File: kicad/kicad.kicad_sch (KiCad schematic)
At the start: 9 parts, among them Q1 BPW40, Q2 BP103BF, U1 PIC16F18875-E/P, U2 L293D

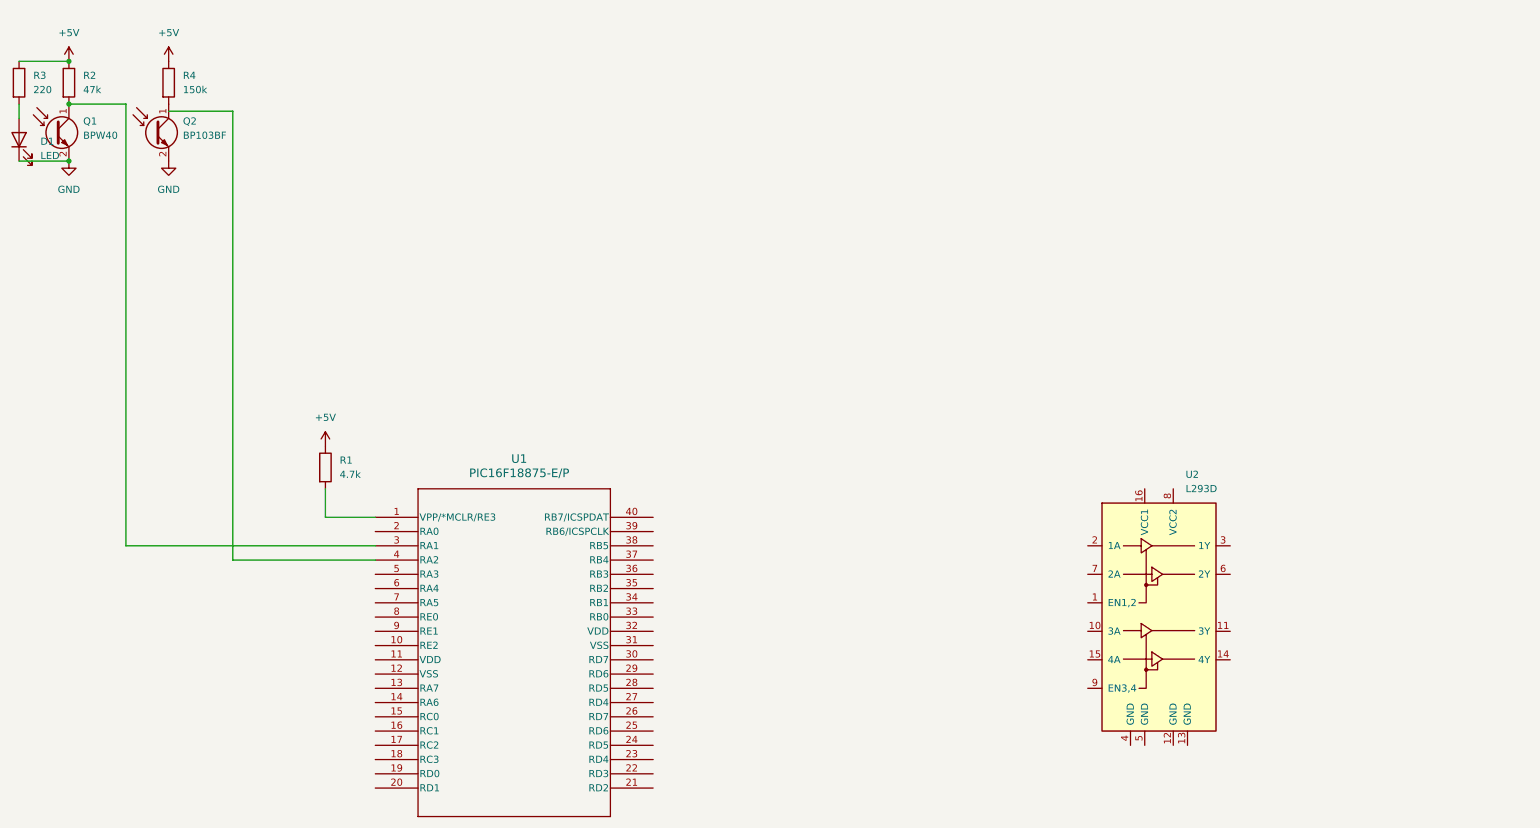
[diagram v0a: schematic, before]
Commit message: finished schematic
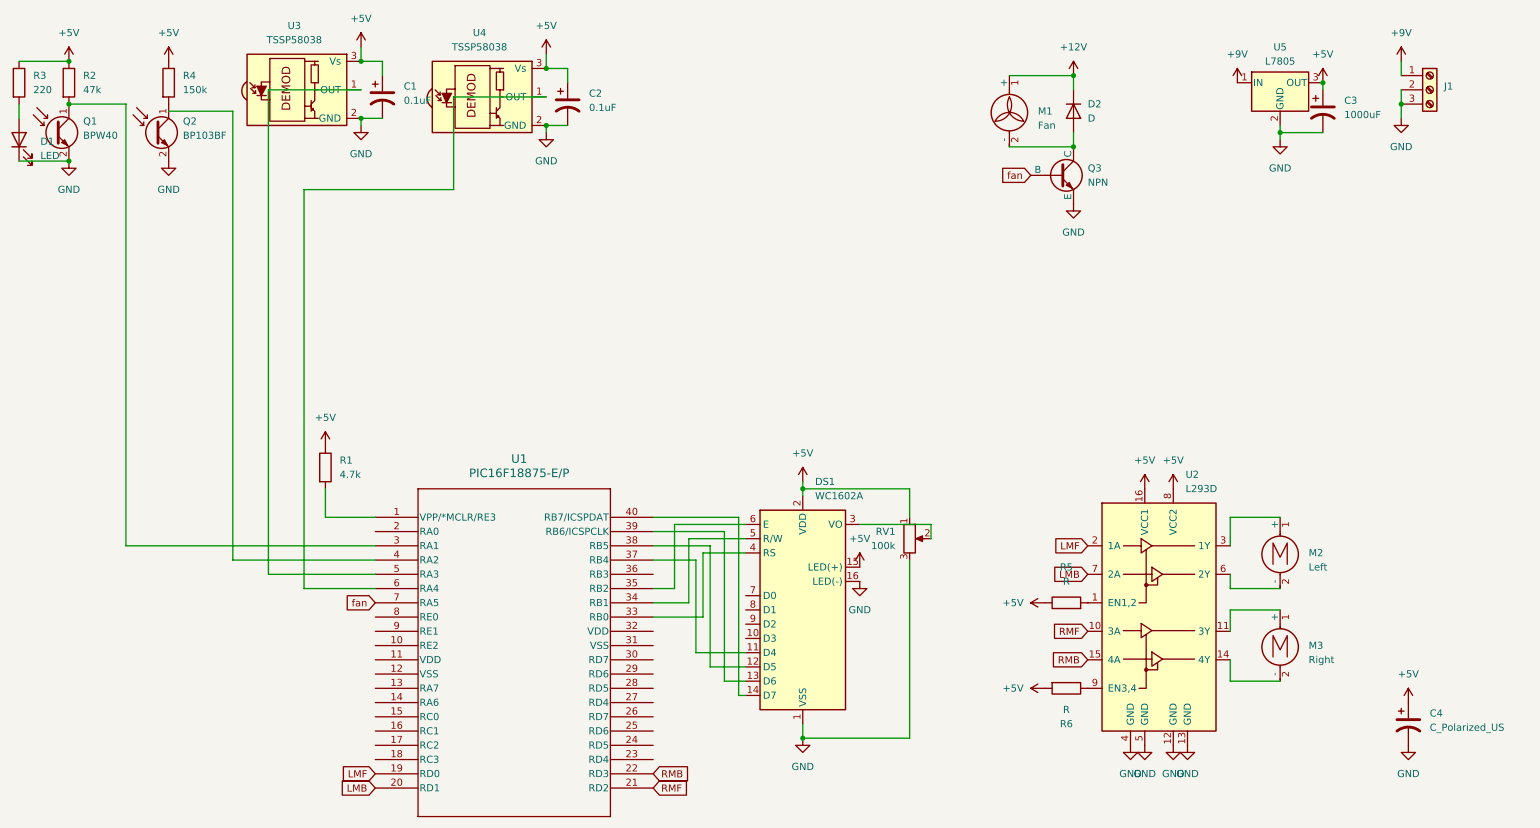
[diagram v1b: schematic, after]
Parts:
- added C1, C2: 0.1uF, symbol Device:C_Polarized_US
- added C3: 1000uF, symbol Device:C_Polarized_US
- added C4: C_Polarized_US, symbol Device:C_Polarized_US
- added D2: D, symbol Device:D
- added DS1: WC1602A, Display:WC1602A, symbol Display_Character:WC1602A
- added J1: ~, symbol Connector:Screw_Terminal_01x03
- added M1: Fan, symbol Motor:Fan
- added M2: Left, symbol Motor:Motor_DC
- added M3: Right, symbol Motor:Motor_DC
- added Q3: NPN, symbol Simulation_SPICE:NPN
- added R5, R6: R, symbol Device:R
- added RV1: 100k, symbol Device:R_Potentiometer
- added U3, U4: TSSP58038, OptoDevice:Vishay_MINICAST-3Pin, symbol Sensor_Proximity:TSSP58038
- added U5: L7805, symbol Regulator_Linear:L7805
- U1: footprint PDIP40_P_MCH -> (none)
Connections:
- net +5V: now also U2.16 (VCC1), U2.8 (VCC2), C1.1, C2.1, C3.1, C4.1, DS1.15 (LED(+)), DS1.2 (VDD), R5.1, R6.2, RV1.1, U3.3 (Vs), U4.3 (Vs), U5.3 (OUT)
- net GND: now also U2.12 (GND), U2.13 (GND), U2.4 (GND), U2.5 (GND), C1.2, C2.2, C3.2, C4.2, DS1.1 (VSS), DS1.16 (LED(-)), J1.2 (Pin_2), J1.3 (Pin_3), Q3.3 (E), RV1.3, U3.2 (GND), U4.2 (GND), U5.2 (GND)
- net at U2.1 (EN1,2): now also R5.2
- net RMF: now reaches U2.10 (3A)
- net RMF: now also U1.21 (RD2)
- net at U2.11 (3Y): now also M3.1 (+)
- net at U2.14 (4Y): now also M3.2 (-)
- net RMB: now reaches U2.15 (4A)
- net RMB: now also U1.22 (RD3)
- net LMF: now reaches U2.2 (1A)
- net LMF: now also U1.19 (RD0)
- net at U2.3 (1Y): now also M2.1 (+)
- net at U2.6 (2Y): now also M2.2 (-)
- net LMB: now reaches U2.7 (2A)
- net LMB: now also U1.20 (RD1)
- net at U2.9 (EN3,4): now also R6.1
- net at U1.33 (RB0): now also DS1.4 (RS)
- net at U1.34 (RB1): now also DS1.5 (R/W)
- net at U1.35 (RB2): now also DS1.6 (E)
- net at U1.37 (RB4): now also DS1.11 (D4)
- net at U1.38 (RB5): now also DS1.12 (D5)
- net at U1.39 (RB6/ICSPCLK): now also DS1.13 (D6)
- net at U1.40 (RB7/ICSPDAT): now also DS1.14 (D7)
- net at U1.5 (RA3): now also U3.1 (OUT)
- net at U1.6 (RA4): now also U4.1 (OUT)
- net fan: now reaches U1.7 (RA5)
- net fan: now also Q3.2 (B)
- new net: D2.2 (A), M1.2 (-), Q3.1 (C)
- new net: DS1.3 (VO), RV1.2
- new net +12V: D2.1 (K), M1.1 (+)
- new net +9V: J1.1 (Pin_1), U5.1 (IN)
